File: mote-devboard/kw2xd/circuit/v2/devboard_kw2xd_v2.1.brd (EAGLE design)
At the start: 41.6 x 55.9 mm, 21 parts, among them J1 CORTEX_DEBUG_PTH, Q1 RED, Q2 RED, Q3 GREEN

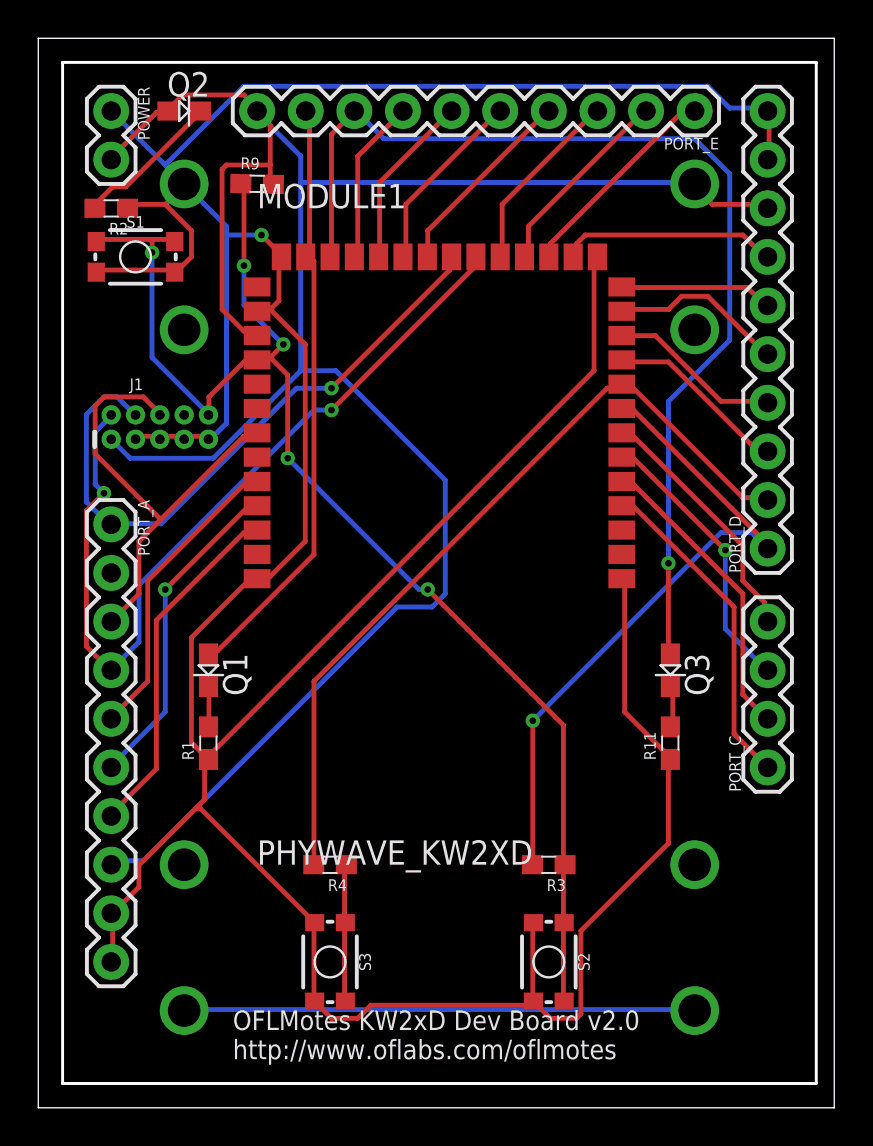
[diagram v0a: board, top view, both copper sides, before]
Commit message: WIP
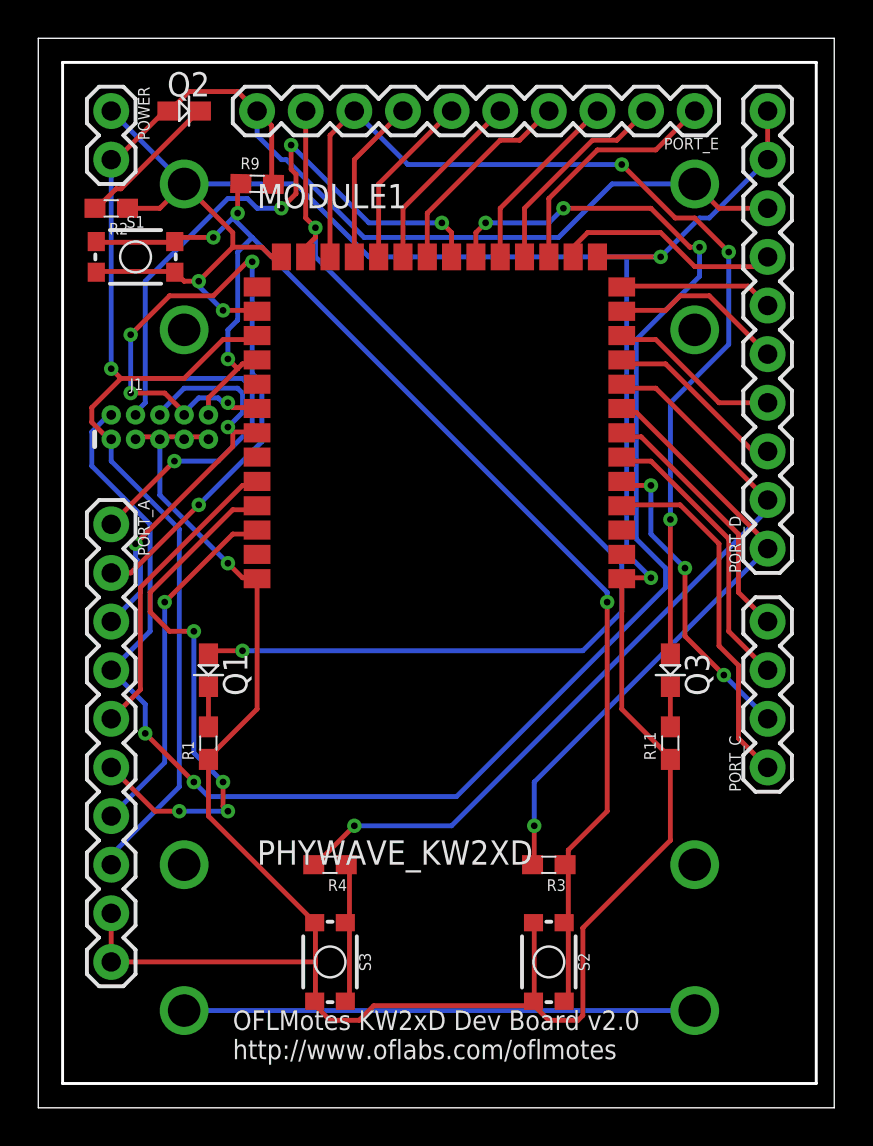
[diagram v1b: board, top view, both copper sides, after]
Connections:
- removed net PTA1: PORT_A.2
- net PTA1_TDI: now also PORT_A.2
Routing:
- net PTA3_SWDIO: track 44.8 -> 87.2 mm, vias 2 -> 5
- net PTA1_TDI: track 0.00 -> 39.2 mm, vias 0 -> 5
- net GND: track 214.3 -> 185.1 mm, vias 1 -> 5
- net PTE19: track 31.3 -> 57.3 mm, vias 0 -> 2
- net VCC: track 117.2 -> 95.0 mm, vias 0 -> 1
- net PTA0_SWDCLK: track 33.6 -> 48.9 mm, vias 1 -> 4
- net PTA18: track 17.1 -> 28.5 mm, vias 1 -> 4
- net PTA2_SWO: track 24.9 -> 21.6 mm, vias 0 -> 2
- net PTE18: track 55.6 -> 53.0 mm, vias 1 -> 3
- net PTD1: track 35.0 -> 32.6 mm
- net PTC4: track 17.2 -> 18.7 mm
- net PTE0: track 11.2 -> 12.6 mm
- net NRST: track 71.1 -> 72.2 mm, vias 5 -> 4
- net PTC5: track 15.8 -> 16.4 mm, vias 0 -> 3
- net PTE1: track 10.4 -> 11.0 mm
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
